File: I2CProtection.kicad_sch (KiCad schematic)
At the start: 9 parts, among them Q7 NX3008NBKS, Q8 MBT2222ADW1T1

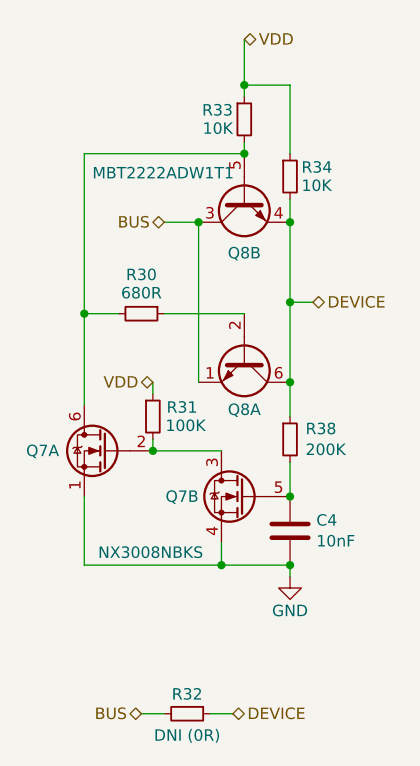
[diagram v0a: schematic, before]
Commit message: Stash
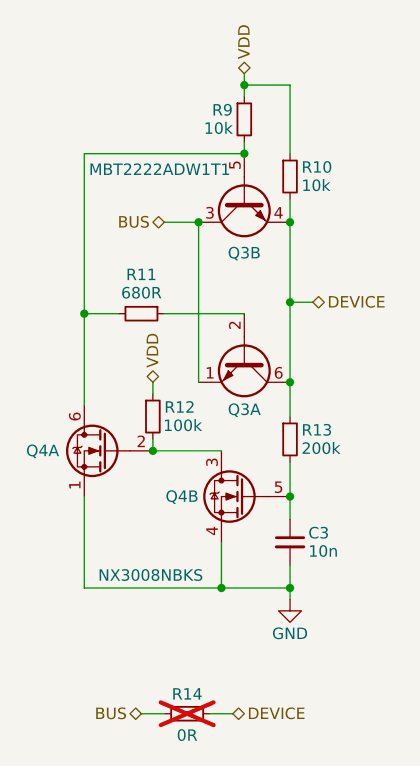
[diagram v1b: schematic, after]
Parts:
- C3: renamed from C4; value 10nF -> 10n; symbol Device:C -> Device:C_Small
- R10: renamed from R34; value 10K -> 10k
- R12: renamed from R31; value 100K -> 100k
- R13: renamed from R38; value 200K -> 200k
- R14: renamed from R32; value DNI (0R) -> 0R; now not fitted; now left out of the parts list
- R9: renamed from R33; value 10K -> 10k
- renumbered Q8 to Q3, Q7 to Q4, R30 to R11
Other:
- company: (none) -> N. Khera
- title: (none) -> Argus -Z Panel
- moved on the sheet: C3
